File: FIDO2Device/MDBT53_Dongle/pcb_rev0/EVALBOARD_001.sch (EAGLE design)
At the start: 47 parts, among them CN1 IF_6PIN, CN2 USB4105-GF-A, CN3 IF_7PIN, SW1 SKRPACE010, SW2 SKTADAE010, U1 MDBT53, U2 XC6206P332MR-G, U3 RV-3028-C7, X1 NX3215SA-32.768K-STD-MUA-9

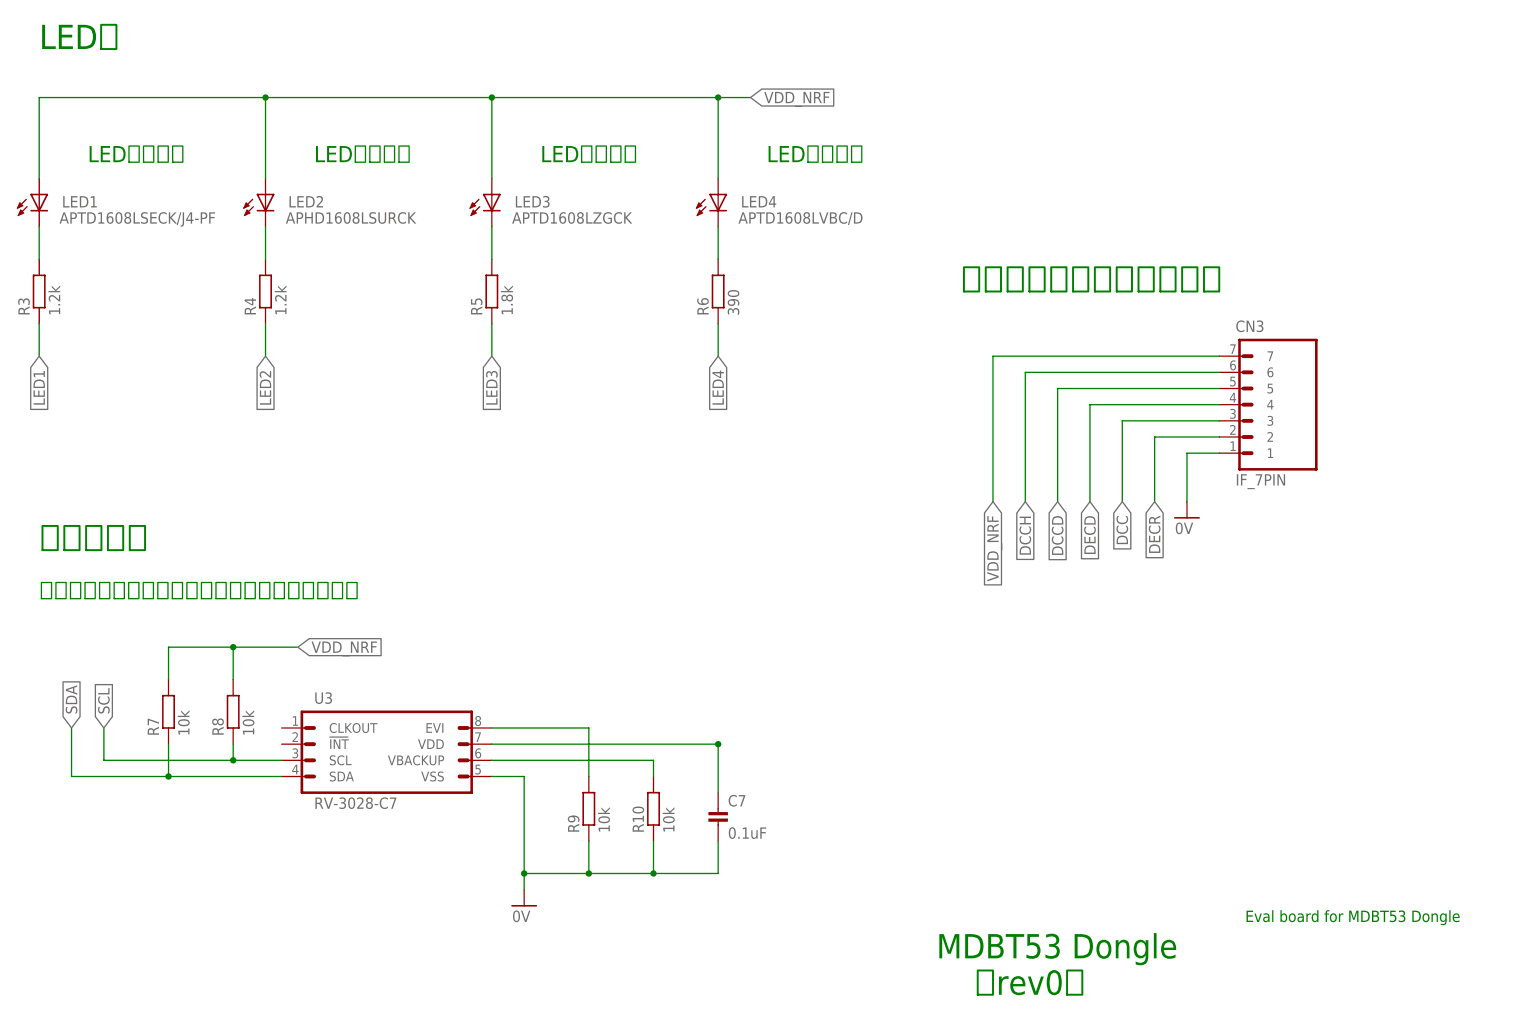
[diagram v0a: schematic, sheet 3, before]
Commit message: 回路図を作成
・部品番号を修正
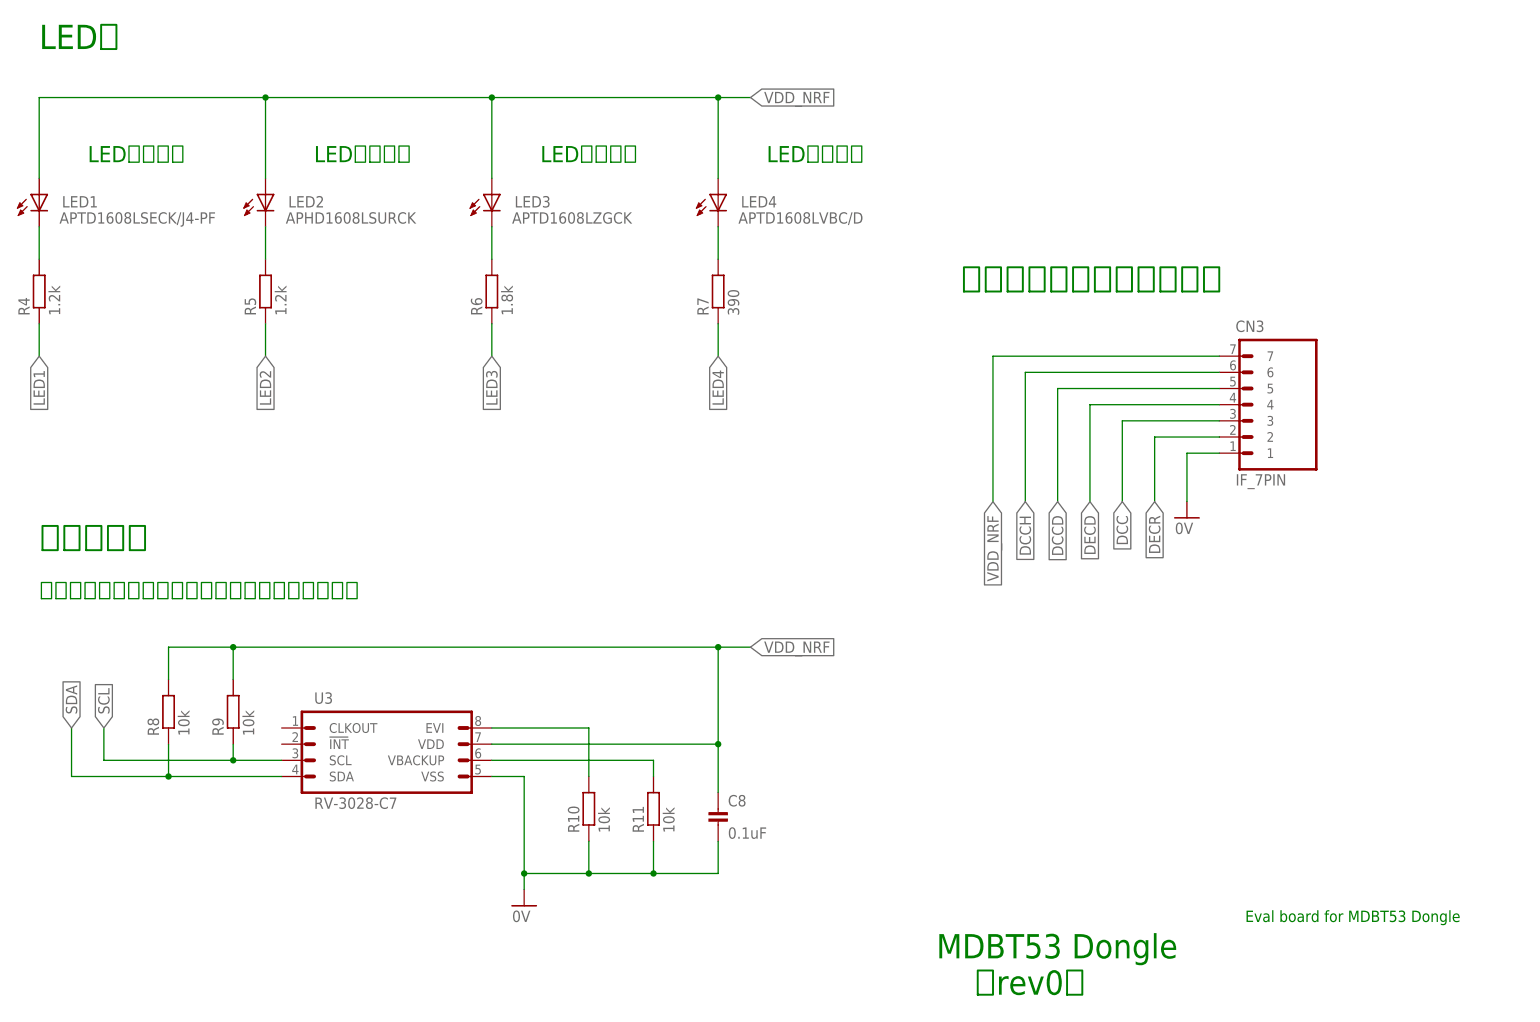
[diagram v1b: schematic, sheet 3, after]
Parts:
- removed L4: BLM15AG121SN1D, Parts:BLM15AG121SN1D
- added L1: BLM15AG121SN1D, Parts:BLM15AG121SN1D
- C10: value 4.7uF -> 1uF
- C7: value 0.1uF -> 4.7uF; device Parts:CAP_0402K -> Parts:CAP_0603
- C8: value 1uF -> 0.1uF; device Parts:CAP_0603 -> Parts:CAP_0402K
- CN1: value IF_6PIN -> USB4105-GF-A; device Connectors:IF_6PIN -> Connectors:USB4105-GF-A
- CN2: value USB4105-GF-A -> IF_6PIN; device Connectors:USB4105-GF-A -> Connectors:IF_6PIN
- R11: value 2.2 -> 10k
- R3: value 1.2k -> 2.2
- R5: value 1.8k -> 1.2k
- R6: value 390 -> 1.8k
- R7: value 10k -> 390
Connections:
- removed net VBATT: C7.1, U3.VDD
- net 0V: now also CN2.1, L2.2, R11.1; no longer CN1.1, L4.2, R9.1
- net D_N: now also CN1.D_N1, CN1.D_N2; no longer CN2.D_N1, CN2.D_N2
- net D_P: now also CN1.D_P1, CN1.D_P2; no longer CN2.D_P1, CN2.D_P2
- net FG: now also CN1.FG1, CN1.FG2, CN1.FG3, CN1.FG4, L3.1; no longer CN2.FG1, CN2.FG2, CN2.FG3, CN2.FG4, L4.1
- net LED1: now also R4.1; no longer R3.1
- net LED2: now also R5.1; no longer R4.1
- net LED3: now also R6.1; no longer R5.1
- net LED4: now also R7.1; no longer R6.1
- net N$1: now also R7.2; no longer R6.2
- net N$10: now also R10.2; no longer R9.2
- net N$2: now also CN1.CC1; no longer CN2.CC1
- net N$3: now also CN1.CC2; no longer CN2.CC2
- net N$6: now also R6.2; no longer R5.2
- net N$7: now also R5.2; no longer R4.2
- net N$8: now also R4.2; no longer R3.2
- net N$9: now also R11.2; no longer R10.2
- net RESET: now also CN2.5; no longer CN1.5
- net SCL: now also R9.1; no longer R8.1
- net SDA: now also R8.1; no longer R7.1
- net SWDCLK: now also CN2.4; no longer CN1.4
- net SWDIO: now also CN2.3; no longer CN1.3
- net TXD: now also CN2.6; no longer CN1.6
- net USB_GND: now also CN1.GND1, CN1.GND2, L2.1; no longer CN2.GND1, CN2.GND2, L3.1
- net VBUS: now also CN1.VBUS1, CN1.VBUS2, L1.1; no longer CN2.VBUS1, CN2.VBUS2, L2.1
- net VBUS_CONN: now also L1.2, R12.1, R3.1; no longer L2.2, R11.1, R13.1
- net VBUS_LDO: now also C9.1, R12.2; no longer C8.1, R13.2
- net VBUS_NRF: now also C7.1, R3.2; no longer C10.1, R11.2
- net VDDH: now also R13.2; no longer R12.2
- net VDD_3V3: now also C10.1; no longer C9.1
- net VDD_NRF: now also C8.1, CN2.2, R13.1, R9.2, U3.VDD; no longer CN1.2, R12.1, R7.2
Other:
- moved on the sheet: C9, L2, L3, R10, R12, R13, R4, R5, R6, R7, R8, R9
